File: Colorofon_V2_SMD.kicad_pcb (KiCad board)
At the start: 2 copper layers, 104 x 94 mm, 94 parts, among them J1 Barrel_Jack_MountingPin, J2 AudioJack3, J3 691322310002, J4 691322310002, J5 691322310002, Q1 BC547, Q2 BC547, Q3 BC547, Q4 PMV65XP, Q5 PMV65XP, Q6 PMV65XP, SW1 SW_Push, U1 LM358, U2 MCP6002-xP, U3 MCP6002-xP

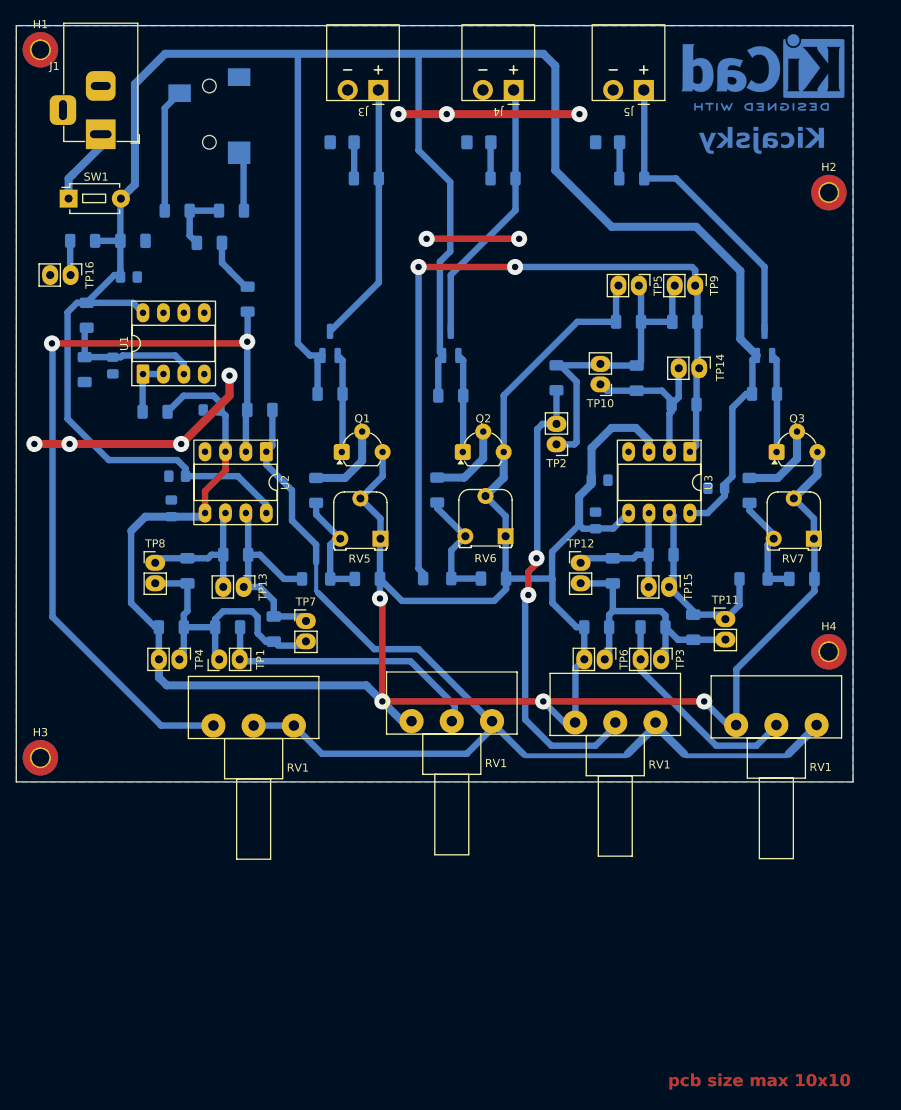
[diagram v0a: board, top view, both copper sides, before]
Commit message: Update layout
Final layout for version 2
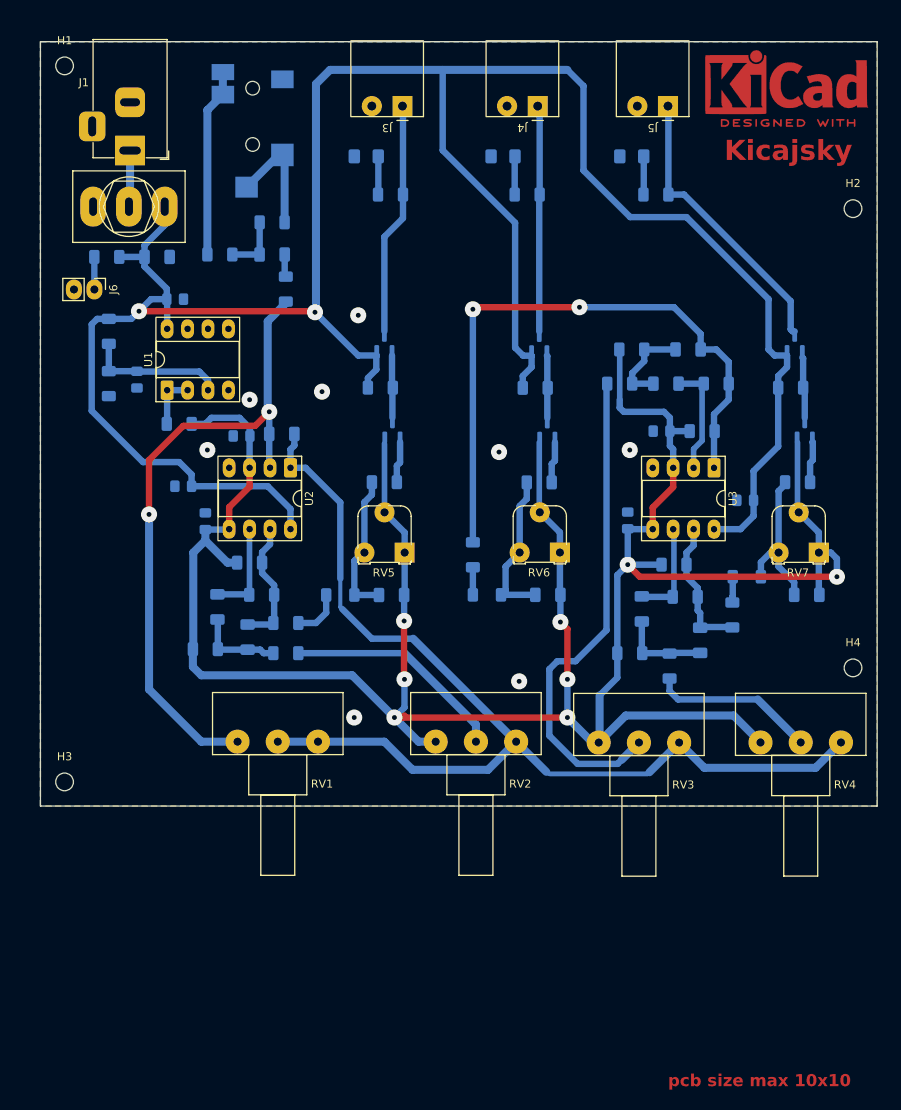
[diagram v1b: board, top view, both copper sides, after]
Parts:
- removed R3: 0/10, Resistor_SMD:R_1206_3216Metric_Pad1.30x1.75mm_HandSolder
- removed the RV1 at (186.5, 134.9)
- removed the RV1 at (146.1, 134.4)
- removed the RV1 at (166.4, 134.6)
- removed SW1: SW_Push, Button_Switch_THT:SW_PUSH_1P1T_6x3.5mm_H4.3_APEM_MJTP1243
- removed SYM1: SYM_EasterEgg_42x60mm, Symbol:KiCad-Logo2_8mm_Copper
- removed TP1, TP10, TP11, TP12, TP13, TP14, TP15, TP16, TP2, TP3, TP4, TP5, TP6, TP7, TP8, TP9: ~, My_Library:PinHeader_1x02_P2.54mm_Vertical_Hand_Solder
- added J6: Conn_01x02_Pin, My_Footprints:PinHeader_1x02_P2.54mm_Vertical_Hand_Solder, F.Cu at (106.7, 80.8)
- added R20: 10, Resistor_SMD:R_1206_3216Metric_Pad1.30x1.75mm_HandSolder, B.Cu at (130.5, 122.2)
- added R22: 1k, Resistor_SMD:R_1206_3216Metric_Pad1.30x1.75mm_HandSolder, B.Cu at (178.8, 115.0)
- added R24: 1k, Resistor_SMD:R_1206_3216Metric_Pad1.30x1.75mm_HandSolder, B.Cu at (182.2, 98.4)
- added R29: 1k, Resistor_SMD:R_1206_3216Metric_Pad1.30x1.75mm_HandSolder, B.Cu at (126.0, 114.8)
- added R30: 10, Resistor_SMD:R_1206_3216Metric_Pad1.30x1.75mm_HandSolder, B.Cu at (153.8, 113.8)
- added R31: 10, Resistor_SMD:R_1206_3216Metric_Pad1.30x1.75mm_HandSolder, B.Cu at (186.0, 121.2)
- added R32: 10, Resistor_SMD:R_1206_3216Metric_Pad1.30x1.75mm_HandSolder, B.Cu at (117.2, 97.5)
- added REF**: KiCad-Logo2_8mm_Copper, Symbol:KiCad-Logo2_8mm_Copper, F.Cu at (192.8, 55.0)
- added RV2: 1k, My_Footprints:Potentiometer_Piher_T-16H_Single_Horizontal, F.Cu at (149.1, 137.0)
- added RV3: 1k, My_Footprints:Potentiometer_Piher_T-16H_Single_Horizontal, F.Cu at (169.4, 137.1)
- added RV4: 1k, My_Footprints:Potentiometer_Piher_T-16H_Single_Horizontal, F.Cu at (189.5, 137.1)
- added SW2: SW_SPDT, My_Footprints:SW_Toggle_Blue_wSlots, F.Cu at (111.0, 70.5)
- C10: value 4,7n -> 680p
- C11: value 4,7n -> 1n
- C12: value 680p -> 100p
- C13: value 680p -> 4,7n
- C17, C18, C19: value 4.7u -> 10u
- C8: value 22n -> 10n
- C9: value 22n -> 33n
- H1, H2, H3, H4: footprint MountingHole:MountingHole_2.2mm_M2_Pad_TopBottom -> MountingHole:MountingHole_2.2mm_M2
- J1: footprint My_Library:BarrelJack_Horizontal -> My_Footprints:BarrelJack_Horizontal
- J2: value AudioJack3 -> AudioJack3_SwitchTR; footprint Connector_Audio:Jack_3.5mm_CUI_SJ-3523-SMT_Horizontal -> My_Footprints:Jack_3.5mm_CUI_SJ2-3593D-SMT_Horizontal
- J3, J4, J5: value 691322310002 -> Connector 1x2 WE 691322310002; footprint My_Library:J_Wurth_WR-TBL_691322310002 -> My_Footprints:J_Wurth_WR-TBL_691322310002
- Q1, Q2, Q3: value BC547 -> BC847; footprint My_Library:TO-92L_Wide_Hand -> Package_TO_SOT_SMD:SOT-23; moved to B.Cu
- Q4, Q5, Q6: footprint Package_TO_SOT_SMD:SOT-23_Handsoldering -> Package_TO_SOT_SMD:SOT-23
- R11: value 1k -> 10k
- R13: value 1M -> 560k
- R14: value 220k -> 660k
- R4, R5, R6: value 5.1k -> 5,1k
- R7: value 56k -> 1k
- R8: value 15k -> 1k
- R9: value 27k -> 1k
- RV1: value 200k -> 100k; footprint My_Library:Potentiometer_Piher_T-16H_Single_Horizontal -> My_Footprints:Potentiometer_Piher_T-16H_Single_Horizontal
- RV5, RV6, RV7: footprint My_Library:Potentiometer_Runtron_RM-065_Vertical_Hand_Solder -> My_Footprints:Potentiometer_Runtron_RM-065_Vertical_Hand_Solder
- U2, U3: value MCP6002-xP -> LM358
- moved R17 12.7 mm to (162.0, 104.8), turned to 0 degrees
- moved Q5 11.0 mm to (162.0, 87.5)
- moved Q2 10.8 mm to (163.0, 98.3), turned to 90 degrees
- moved R21 10.5 mm to (161.5, 93.0)
- moved C15 9.82 mm to (177.2, 98.4), turned to 0 degrees
- moved R16 8.54 mm to (142.8, 104.8), turned to 0 degrees
- moved C3 7.93 mm to (128.8, 76.5)
- moved R7 7.92 mm to (130.5, 126.0)
- moved R8 7.89 mm to (172.0, 92.5), turned to 0 degrees
- moved R5 7.60 mm to (122.3, 76.5)
- moved C18 7.05 mm to (163.1, 118.8)
- moved RV6 7.05 mm to (164.6, 113.5)
- moved Q1 6.87 mm to (143.8, 98.2), turned to 90 degrees
- moved Q4 6.75 mm to (142.8, 87.5)
- moved D2 6.50 mm to (155.5, 118.8)
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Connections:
- C10 pad 1: Net-(D2-A) -> Net-(C10-Pad1)
- C12 pad 1: Net-(D3-A) -> Net-(C12-Pad1)
- C8 pad 1: Net-(D1-A) -> Net-(C8-Pad1)
- Q1 pad 1: Net-(Q1-C) -> Net-(Q1-B)
- Q1 pad 2: Net-(Q1-B) -> /Vref
- Q1 pad 3: /Vref -> Net-(Q1-C)
- Q2 pad 1: Net-(Q2-C) -> Net-(Q2-B)
- Q2 pad 2: Net-(Q2-B) -> /Vref
- Q2 pad 3: /Vref -> Net-(Q2-C)
- Q3 pad 1: Net-(Q3-C) -> Net-(Q3-B)
- Q3 pad 2: Net-(Q3-B) -> /Vref
- Q3 pad 3: /Vref -> Net-(Q3-C)
- R13 pad 2: Net-(D1-A) -> Net-(C8-Pad1)
- R14 pad 2: Net-(D2-A) -> Net-(C10-Pad1)
- R15 pad 2: Net-(D3-A) -> Net-(C12-Pad1)
- U1 pad 5: unconnected-(U1B-+-Pad5) -> GND
- U1 pad 6: unconnected-(U1B---Pad6) -> GND
- U2 pad 7: Net-(D1-A) -> Net-(C8-Pad1)
- U3 pad 1: Net-(D2-A) -> Net-(C10-Pad1)
- U3 pad 7: Net-(D3-A) -> Net-(C12-Pad1)
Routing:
- net Net-(D2-A): track 95.5 -> 3.43 mm, vias 2 -> 0
- net Net-(C10-Pad1): track 0.00 -> 78.8 mm, vias 0 -> 2
- net GND: track 63.4 -> 0.00 mm, vias 9 -> 8
- net Net-(C10-Pad2): track 40.6 -> 11.4 mm
- net Net-(C8-Pad2): track 36.6 -> 10.8 mm
- net Net-(C12-Pad2): track 34.4 -> 11.0 mm
- net Net-(D1-A): track 27.7 -> 6.21 mm
- net Net-(D3-A): track 24.2 -> 3.22 mm
- net Net-(U2A--): track 101.3 -> 81.2 mm
- net Net-(C12-Pad1): track 0.00 -> 17.0 mm
- net /Vref: track 336.4 -> 320.2 mm, vias 4 -> 8
- net Net-(C8-Pad1): track 0.00 -> 15.6 mm
- net +12V: track 309.5 -> 295.9 mm, vias 0 -> 2
- net Net-(J2-PadR): track 15.4 -> 23.5 mm
- net Net-(J2-PadT): track 6.35 -> 13.8 mm
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- added copper zone on F.Cu, net GND
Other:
- board size 104 x 94 mm -> 104 x 95 mm
